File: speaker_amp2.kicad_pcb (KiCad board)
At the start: 2 copper layers, 99 x 85 mm, 74 parts, among them J1 Molex_430450227, J2 Molex_430450227, J3 Molex_430450227, J4 Molex_430450227, J5 Molex_1053101106, J6 Molex_430450227, U1 TAS5822MDCPR, U2 TAS5822MDCPR

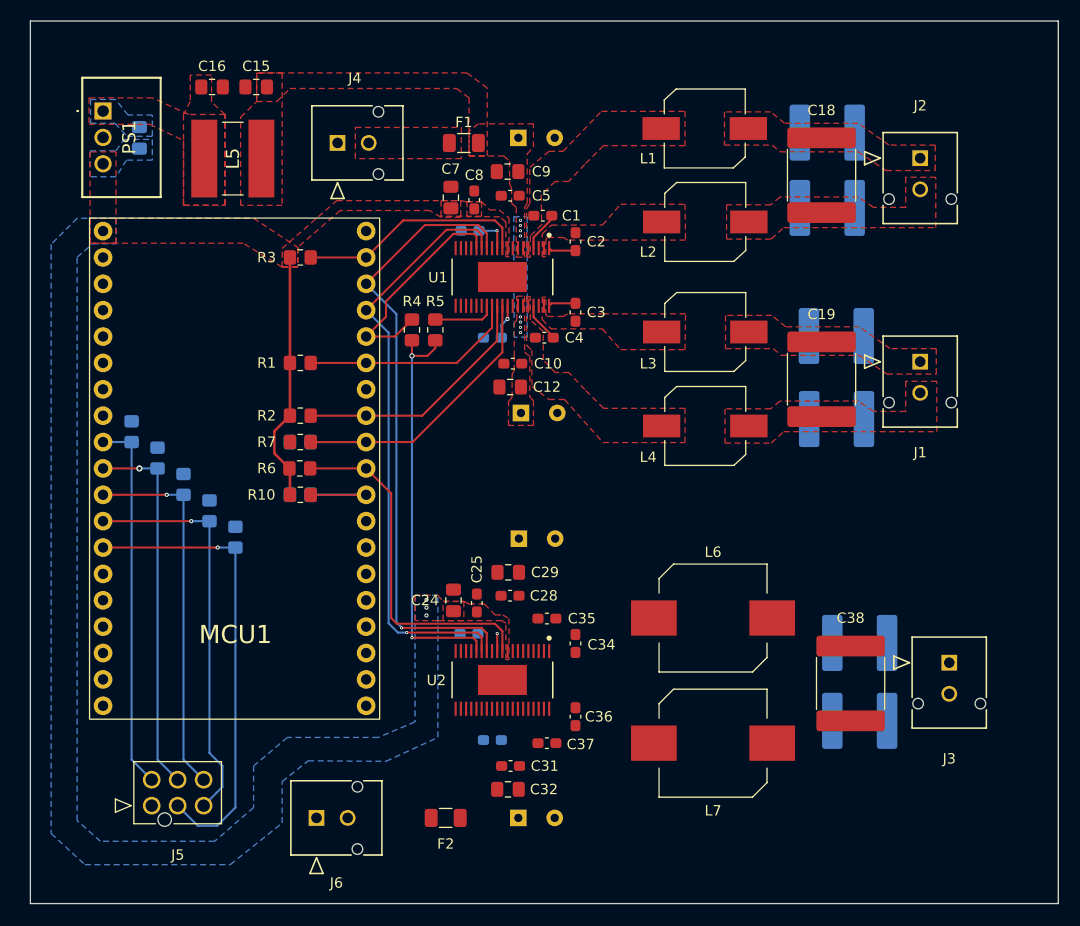
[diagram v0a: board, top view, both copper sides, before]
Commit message: first finalized pcb
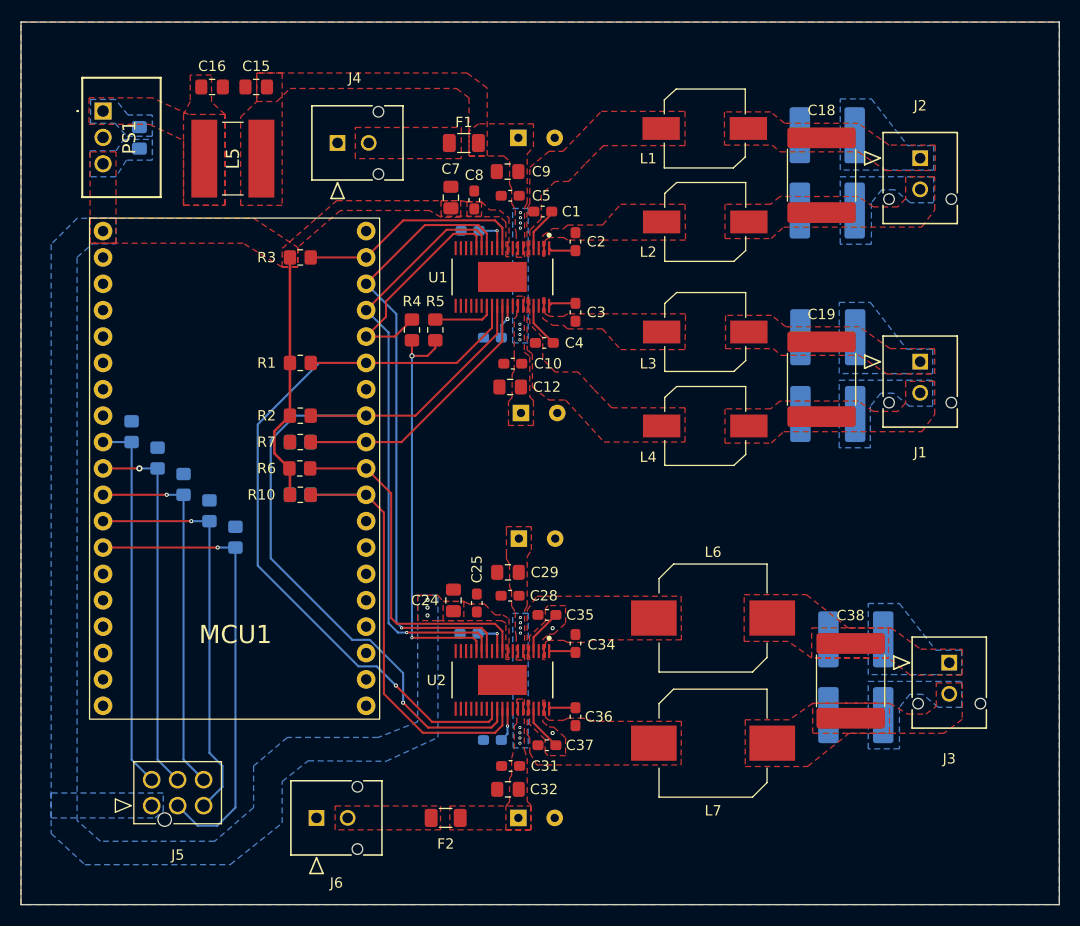
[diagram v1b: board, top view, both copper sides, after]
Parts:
- moved C23 0.98 mm to (116.0, 102.8)
- moved C21 0.83 mm to (116.0, 95.5)
- moved C39 0.66 mm to (118.8, 131.8)
- moved C40 0.51 mm to (118.8, 124.5)
- moved C4 0.50 mm to (88.8, 96.0)
- moved C1 0.40 mm to (88.6, 83.3)
- moved C35 0.35 mm to (89.0, 122.2), turned to 180 degrees
- moved C20 0.25 mm to (116.0, 83.2)
- moved C22 0.25 mm to (116.0, 76.0)
- moved C38 0.25 mm to (118.2, 128.6)
- moved C37 0.20 mm to (89.0, 134.8), turned to 0 degrees
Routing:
- net /SDA: track 21.0 -> 77.3 mm, vias 0 -> 1
- net /SCL: track 24.3 -> 77.2 mm, vias 0 -> 1
- net /PDN2: track 10.7 -> 45.4 mm
- net Net-(U2-BST_B+): track 0.00 -> 4.40 mm
- net Net-(U2-BST_A+): track 0.00 -> 4.38 mm
- net Net-(U2-AVDD): track 0.00 -> 3.26 mm, vias 0 -> 1
- net Net-(U2-BST_A-): track 0.00 -> 2.59 mm
- net Net-(U2-BST_B-): track 0.00 -> 2.58 mm
- net Net-(U2-VR_DIG): track 1.69 -> 3.54 mm
- net /PDN1: track 31.9 -> 31.2 mm
- net PVDD2: vias 0 -> 8
- net GND: vias 0 -> 2
- added copper zone on B.Cu, net GND
- added copper zone on F.Cu, net GND
- added copper zone on B.Cu, net Net-(C18-Pad1)
- added copper zone on B.Cu, net Net-(C18-Pad2)
- added copper zone on B.Cu, net Net-(C19-Pad1)
- added copper zone on B.Cu, net Net-(C19-Pad2)
- added copper zone on B.Cu, net Net-(C38-Pad1)
- added copper zone on F.Cu, net Net-(C38-Pad1)
- added copper zone on B.Cu, net Net-(C38-Pad2)
- added copper zone on F.Cu, net Net-(C38-Pad2)
- added copper zone on F.Cu, net Net-(F2-Pad2)
- added copper zone on F.Cu, net Net-(U2-OUT_A+)
- added copper zone on F.Cu, net Net-(U2-OUT_B+)
- added copper zone on B.Cu, net PVDD2
- added copper zone on F.Cu, net PVDD2
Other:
- board size 99 x 85 mm -> 100 x 85 mm
